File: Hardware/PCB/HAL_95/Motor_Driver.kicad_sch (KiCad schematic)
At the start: 14 parts, among them J2 Conn_01x06, J4 Conn_01x06, J5 SERVO, U2 DRV8833PWPR

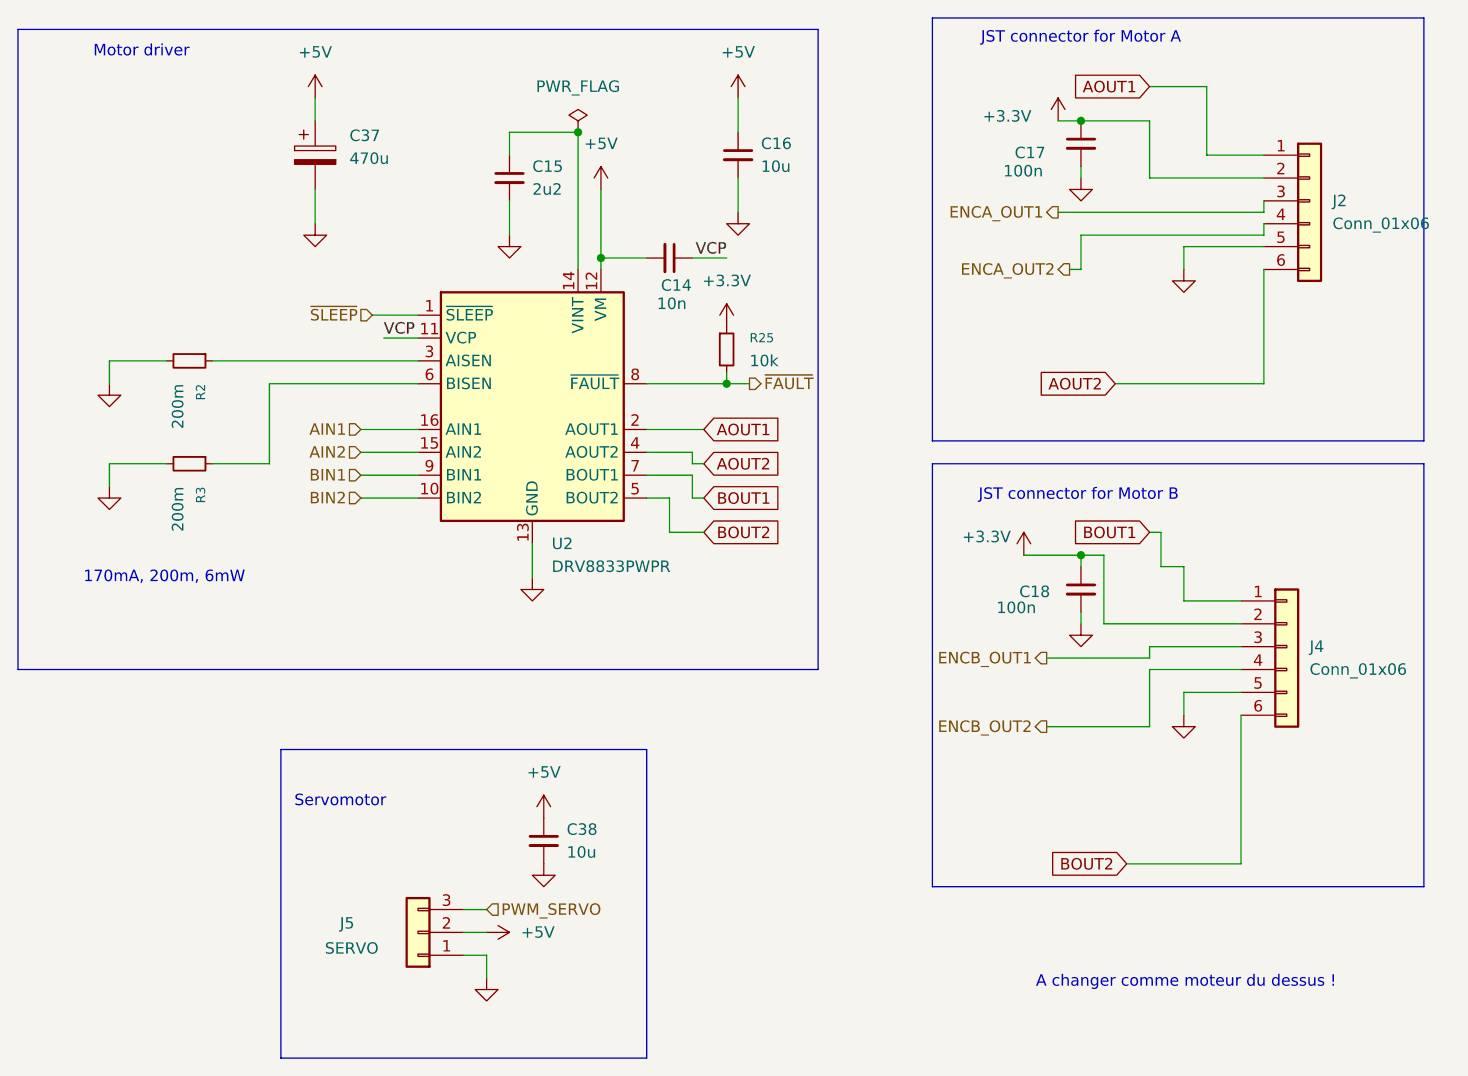
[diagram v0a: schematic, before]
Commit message: removed erc errors
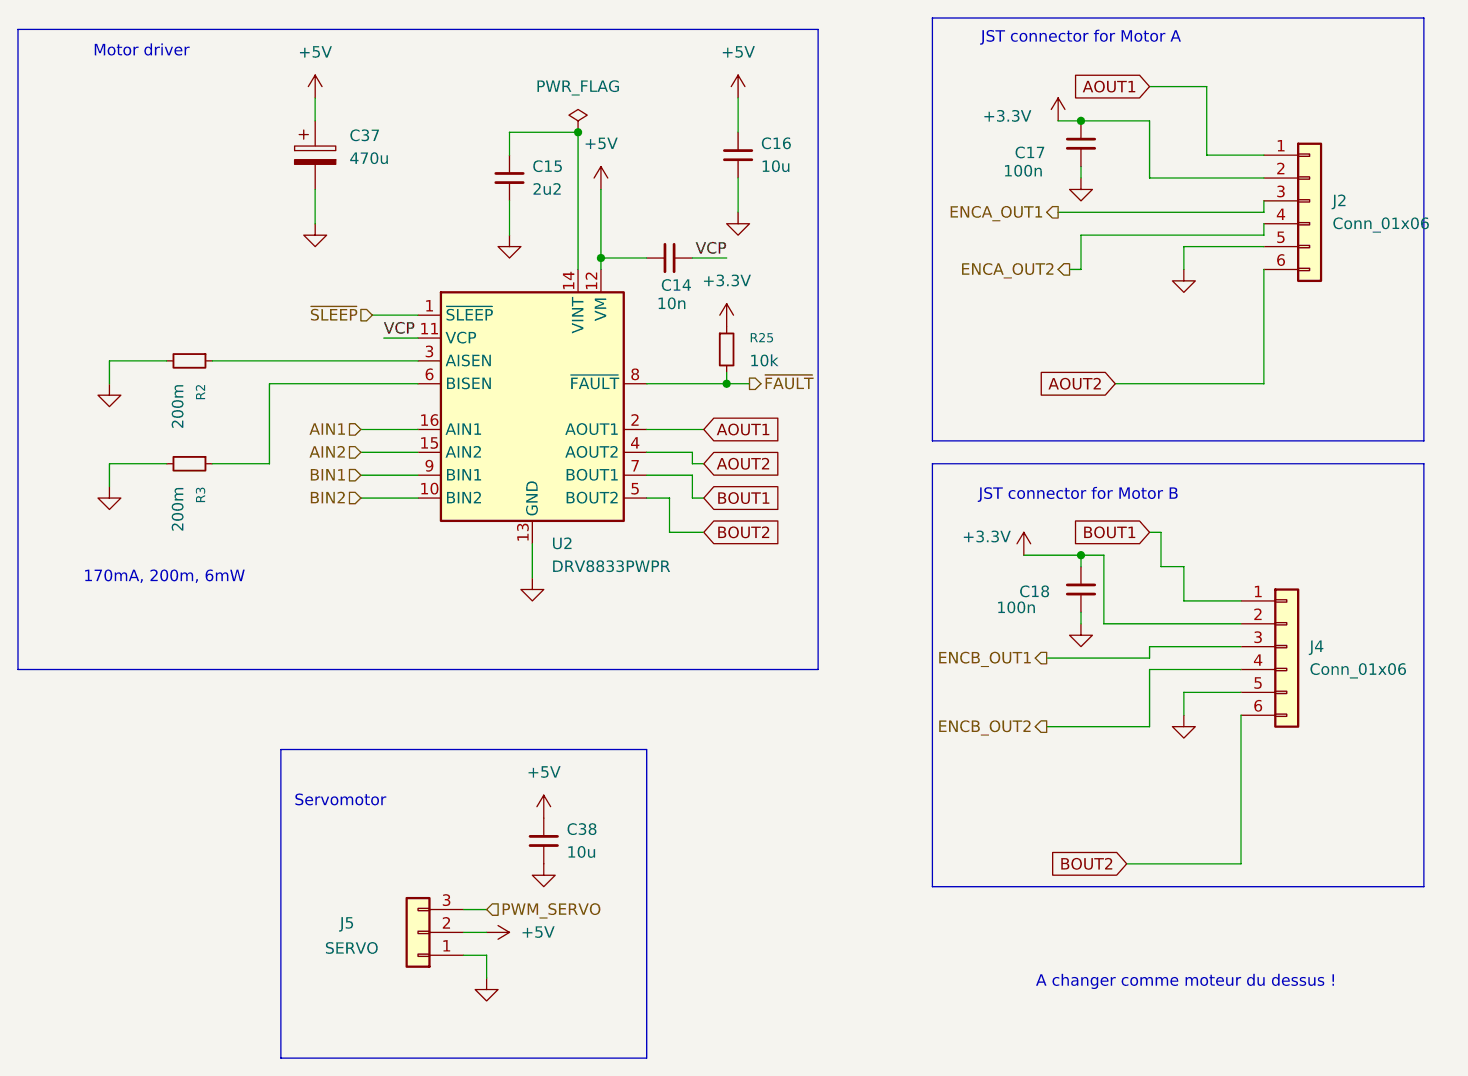
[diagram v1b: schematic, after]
